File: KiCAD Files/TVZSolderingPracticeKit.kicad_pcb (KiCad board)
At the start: 2 copper layers, 100 x 100 mm, 21 parts, among them U1 NE555P

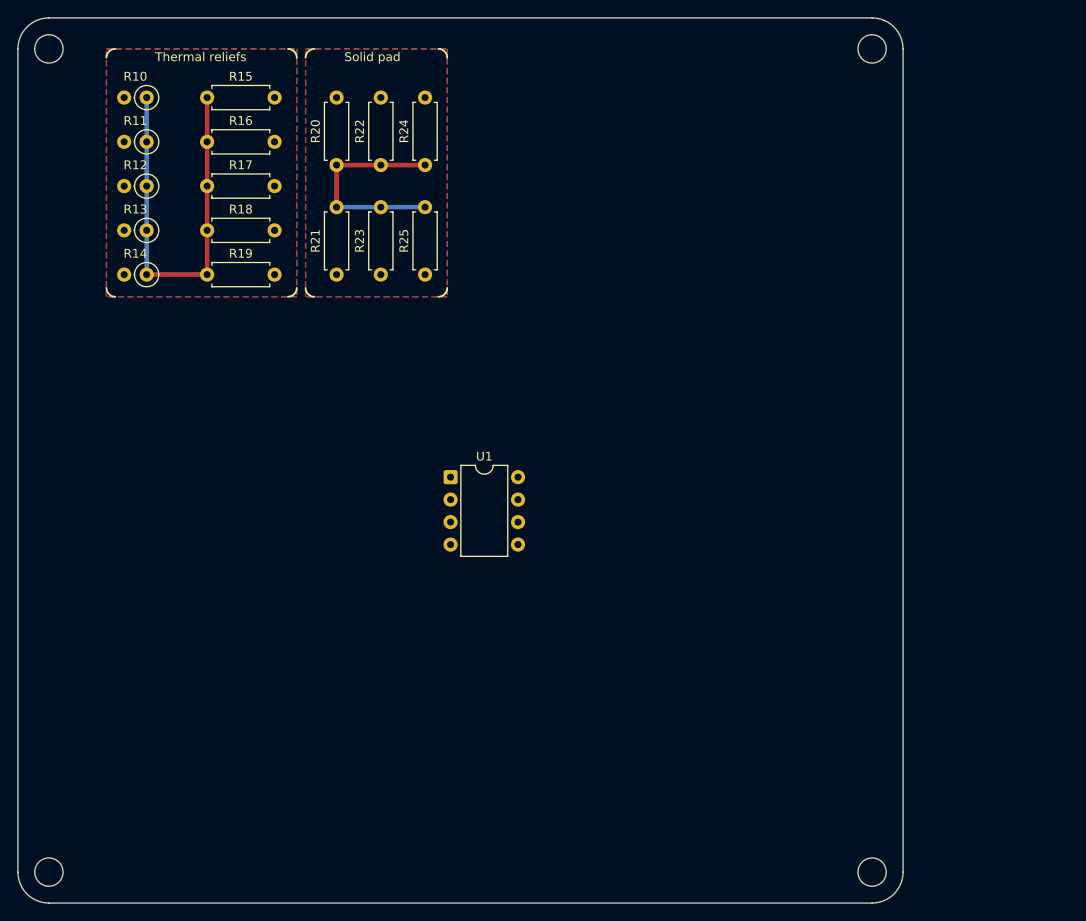
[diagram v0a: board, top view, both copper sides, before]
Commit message: update
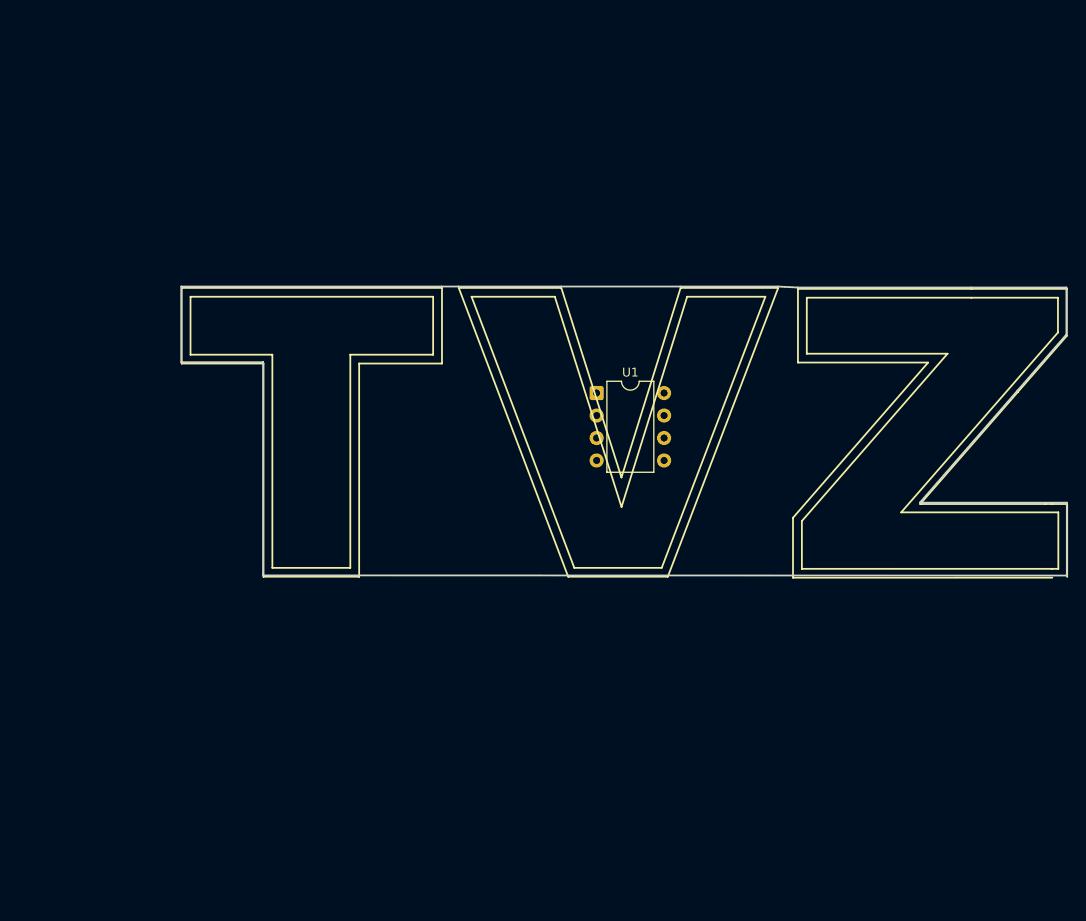
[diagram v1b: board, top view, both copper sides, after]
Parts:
- removed H1, H2, H3, H4: MountingHole, MountingHole:MountingHole_3.2mm_M3
- removed R10, R11, R12, R13, R14: R, Resistor_THT:R_Axial_DIN0207_L6.3mm_D2.5mm_P2.54mm_Vertical
- removed R15, R16, R17, R18, R19, R20, R21, R22, R23, R24, R25: R, Resistor_THT:R_Axial_DIN0207_L6.3mm_D2.5mm_P7.62mm_Horizontal
- moved U1 19.0 mm to (151.9, 88.4)
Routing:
- net Net-(R10-Pad1): track 46.8 -> 0.00 mm
- net Net-(R20-Pad1): track 24.8 -> 0.00 mm
- removed copper zone on B.Cu, net GND2
- removed copper zone on F.Cu, net GND2
- removed copper zone on B.Cu, net GND3
- removed copper zone on F.Cu, net GND3
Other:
- board size 100 x 100 mm -> 100 x 32.7 mm
- board text removed: "Solid pad"
- board text removed: "Thermal reliefs"
